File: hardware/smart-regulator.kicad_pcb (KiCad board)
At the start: 2 copper layers, 157 x 56 mm, 67 parts, among them J2 Conn_02x20_Top_Bottom, P1 USB_A_2, SW1 SW_PUSH, SW2 SW_PUSH, SW3 SW_PUSH, U1 ESP-WROOM-32, U10 Power-Monitor-INA219, U11 DAC, U12 ZLDO1117G33TA, U14 SI7006-A20, U15 TSL45315CL, U2 housing-mounts, U3 LM2576, U4 LM2576, U5 LM2576, U6 LM2576, U7 ACS712ELCTR-05B-T_NRND, U8 Power-Monitor-INA219, U9 Power-Monitor-INA219

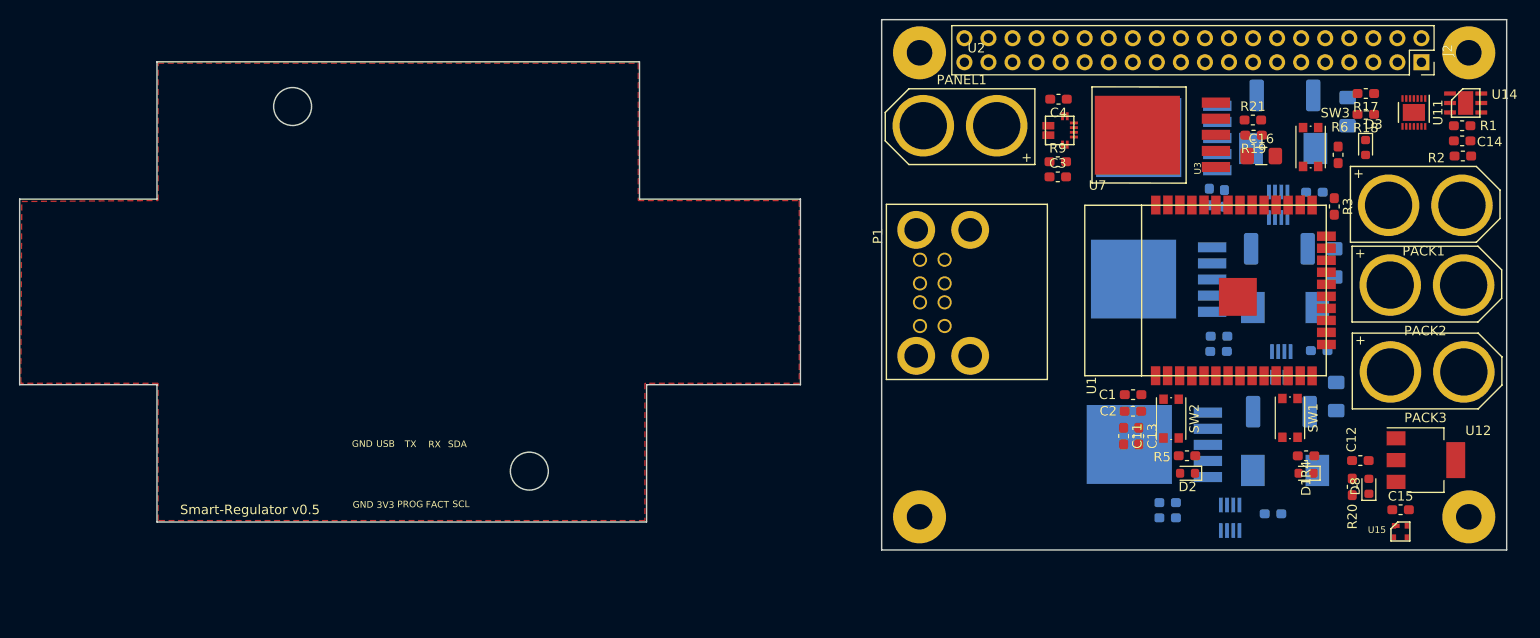
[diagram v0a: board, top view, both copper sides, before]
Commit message: traces complete
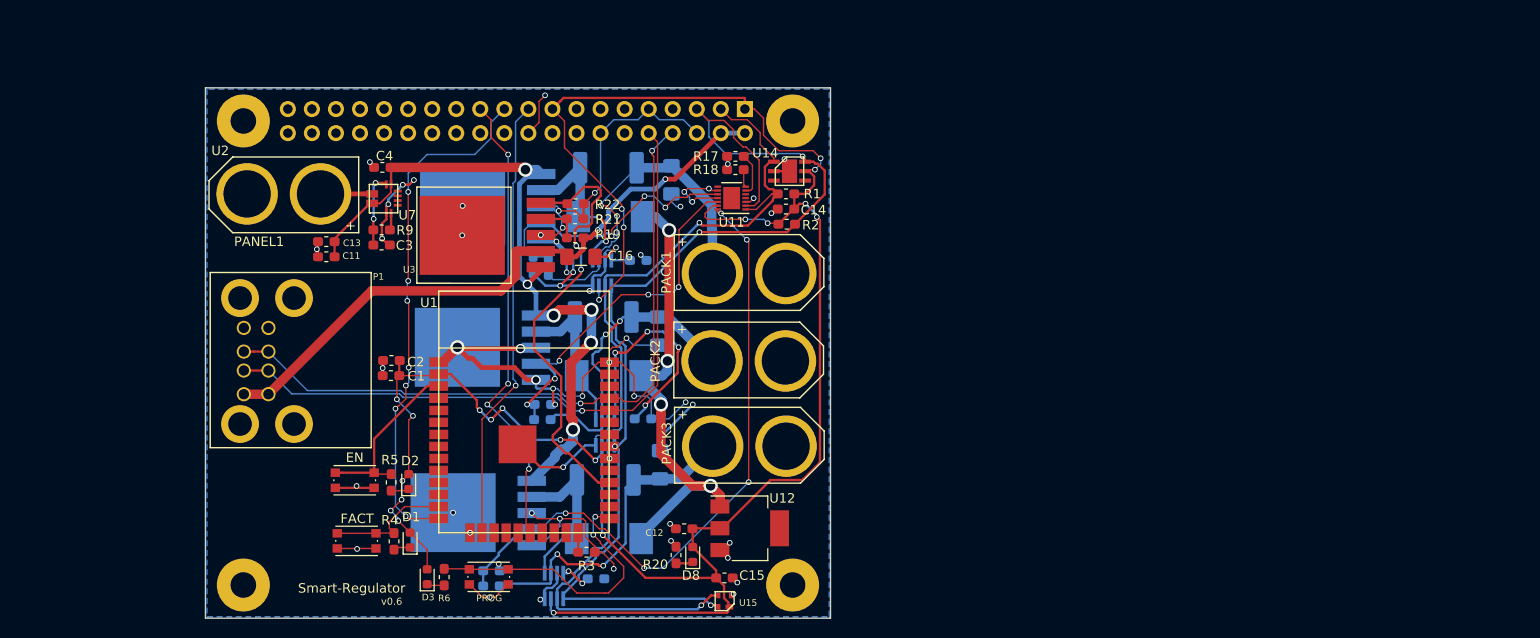
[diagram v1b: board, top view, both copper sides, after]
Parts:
- added LOGO: , open-automation:LOGO, B.Cu at (130.4, 107.8)
- added R22: R_10k, Resistor_SMD:R_0603_1608Metric_Pad1.05x0.95mm_HandSolder, F.Cu at (151.9, 92.6)
- J2: value Conn_02x20_Top_Bottom -> Conn_02x20_Odd_Even; moved to B.Cu
- moved D3 109.0 mm to (136.2, 132.0), turned to 90 degrees
- moved R6 104.4 mm to (138.1, 132.0), turned to 90 degrees
- moved FACT 99.4 mm to (128.8, 128.2), turned to 0 degrees
- moved PROG 97.9 mm to (142.8, 132.0), turned to 0 degrees
- moved R4 96.7 mm to (132.8, 128.2), turned to 90 degrees
- moved D1 94.9 mm to (134.4, 128.1), turned to 90 degrees
- moved C13 88.2 mm to (125.6, 96.6), turned to 180 degrees
- moved R3 87.0 mm to (153.1, 129.4), turned to 180 degrees
- moved EN 86.5 mm to (128.6, 121.8), turned to 0 degrees
- moved C11 86.3 mm to (125.6, 98.2), turned to 180 degrees
- moved R5 84.1 mm to (132.4, 122.0), turned to 90 degrees
- moved D2 82.2 mm to (134.3, 121.9), turned to 90 degrees
- moved C2 78.5 mm to (132.5, 109.2)
- moved C1 78.4 mm to (132.4, 110.8)
- moved U1 77.0 mm to (137.5, 110.6), turned to 0 degrees
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- renumbered SW2 to EN, SW1 to FACT, SW3 to PROG
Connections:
- net /PANEL_SW renamed Net-(U1-Pad27)
- J2 pad 10: Net-(J2-Pad10) -> /RXD
- J2 pad 13: GND -> Net-(J2-Pad13)
- J2 pad 14: Net-(J2-Pad14) -> GND
- J2 pad 17: Net-(J2-Pad17) -> 3V3
- J2 pad 19: Net-(J2-Pad19) -> /microcontroller/MOSI
- J2 pad 2: /SDA -> /V_USB
- J2 pad 21: /V_USB -> /microcontroller/MISO
- J2 pad 22: /V_USB -> Net-(J2-Pad22)
- J2 pad 23: GND -> /microcontroller/SCLK
- J2 pad 24: /TXD -> Net-(J2-Pad24)
- J2 pad 25: /RXD -> GND
- J2 pad 27: GND -> Net-(J2-Pad27)
- J2 pad 3: /SCL -> /SDA
- J2 pad 34: Net-(J2-Pad34) -> GND
- J2 pad 35: GND -> Net-(J2-Pad35)
- J2 pad 37: GND -> Net-(J2-Pad37)
- J2 pad 39: Net-(J2-Pad39) -> GND
- J2 pad 4: Net-(J2-Pad4) -> /V_USB
- J2 pad 5: GND -> /SCL
- J2 pad 6: Net-(J2-Pad6) -> GND
- J2 pad 8: Net-(J2-Pad8) -> /TXD
- J2 pad 9: 3V3 -> GND
- U1 pad 14: Net-(U1-Pad14) -> /microcontroller/MISO
- U1 pad 16: Net-(U1-Pad16) -> /microcontroller/MOSI
- U1 pad 20: Net-(U1-Pad20) -> /microcontroller/SCLK
- U1 pad 28: /POWER_EN -> /USB_EN
- U3 pad 5: GND -> /USB_EN
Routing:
- net 3V3: track 0.00 -> 233.0 mm, vias 0 -> 22
- net GND: track 0.00 -> 220.7 mm, vias 0 -> 57
- net /SCL: track 0.00 -> 116.6 mm, vias 0 -> 4
- net /SDA: track 0.00 -> 98.9 mm, vias 0 -> 3
- net /Power/REG_POWER: track 0.00 -> 75.7 mm, vias 0 -> 6
- net /TXD: track 0.00 -> 74.4 mm, vias 0 -> 2
- net /RXD: track 0.00 -> 73.6 mm, vias 0 -> 1
- net /Power/OUT3: track 0.00 -> 68.7 mm, vias 0 -> 5
- net /V_USB: track 0.00 -> 67.5 mm, vias 0 -> 2
- net /microcontroller/MISO: track 0.00 -> 54.9 mm, vias 0 -> 7
- net /V_MAIN: track 0.00 -> 49.7 mm, vias 0 -> 4
- net /microcontroller/SCLK: track 0.00 -> 49.1 mm, vias 0 -> 4
- net /USB_EN: track 0.00 -> 47.1 mm, vias 0 -> 2
- net /microcontroller/MOSI: track 0.00 -> 47.0 mm, vias 0 -> 1
- net /Power/OUT2: track 0.00 -> 39.5 mm, vias 0 -> 5
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- added copper zone on B.Cu, net GND
- removed copper zone on F.Cu, net GND
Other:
- board size 157 x 56 mm -> 66 x 56 mm
- net class DELETE removed
- net class Default: trace_width 0.25 -> 0.2
- net class x-small added: clearance 0.2, trace_width 0.2, via_dia 0.6, via_drill 0.4
- rule pad_to_mask_clearance: 0.2 -> 0
- rule trace_min: 0.2 -> 0
- board text added: "Smart-Regulator"
- board text added: "v0.6"
- board text removed: "FACT"
- board text removed: "PROG"
- board text removed: "Smart-Regulator v0.5"
